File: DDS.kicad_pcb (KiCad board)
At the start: 4 copper layers, 70 x 100 mm, 175 parts, among them J1 Conn_01x05_Male, J2 USB_B_Mini, J3 Barrel_Jack_Switch, J4 Conn_Coaxial, J5 Conn_Coaxial, J6 Conn_Coaxial, U1 5M160ZT100, U2 LM317_SOT-223, U3 MCP2210x-SS, U4 ETXO-H33CL-100.000, U5 IS61LF12836, U6 DAC5687IPZP, Y1 12Meg

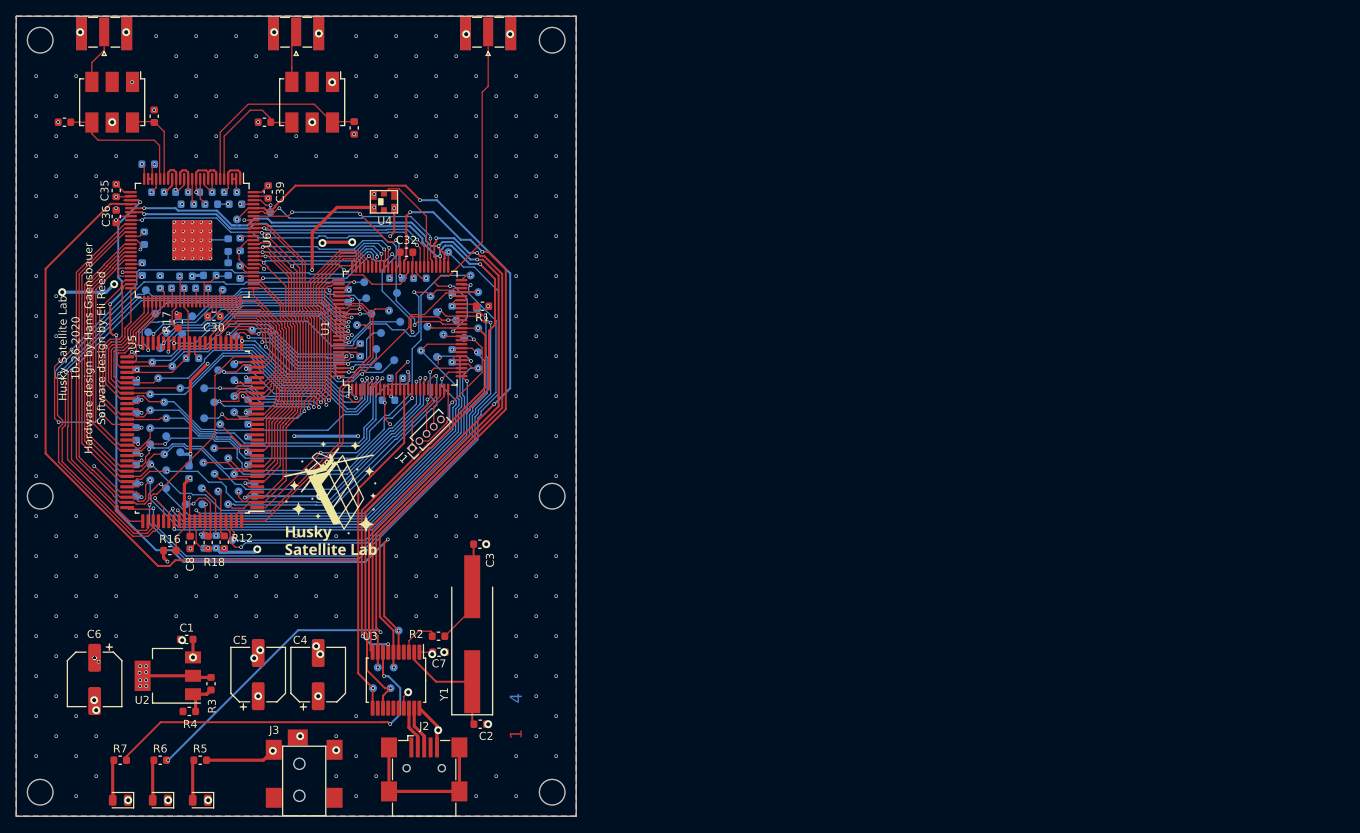
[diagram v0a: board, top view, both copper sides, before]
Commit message: new changes
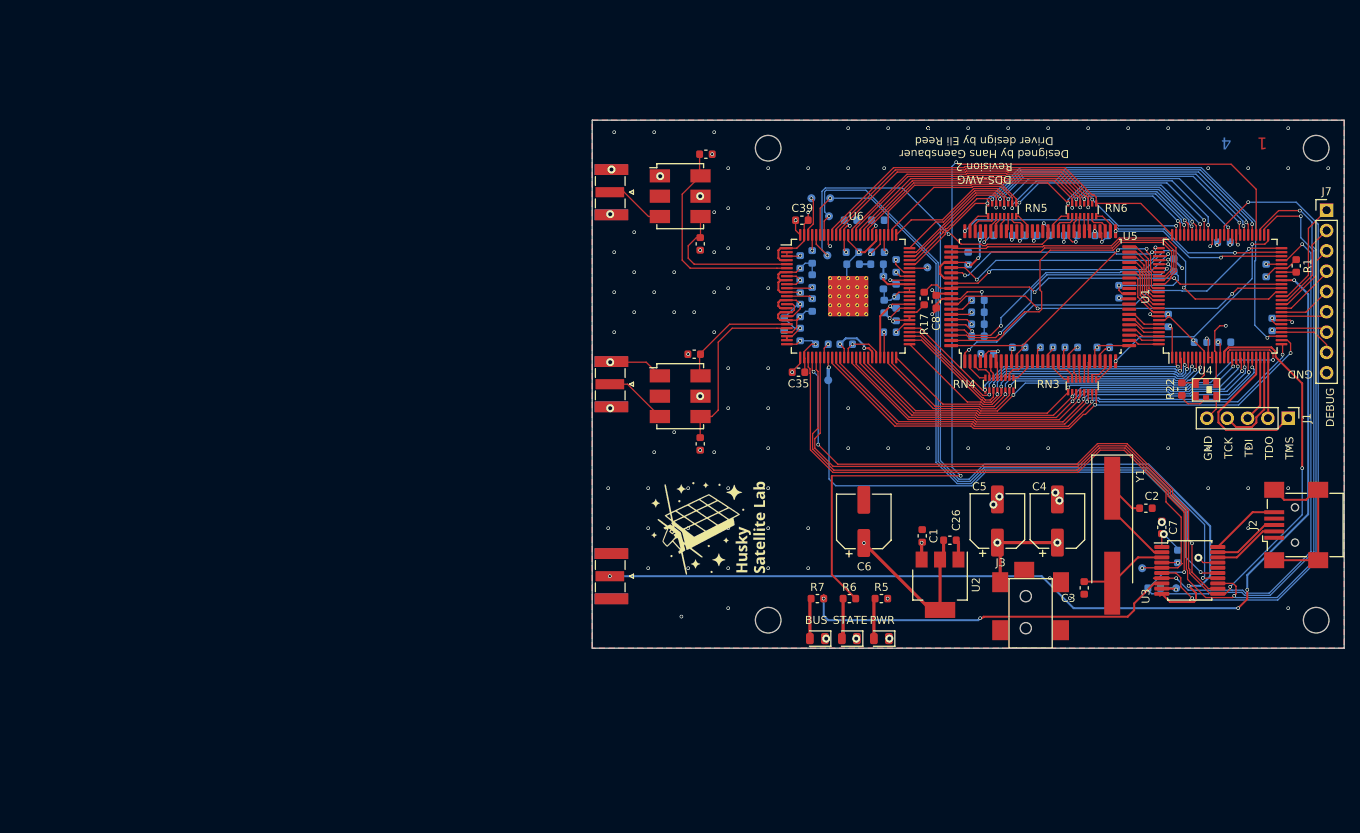
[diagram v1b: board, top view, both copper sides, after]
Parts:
- removed A0, A1, A10, A11, A12, A13, A14, A15, A16, A2, A3, A4, A5, A6, A7, A8, A9, CS_DAC, CS_MEM, D0, D10, D11, D12, D13, D14, D15, D16, D17, D18, D19, D20, D21, D22, D23, D24, D25, D26, D27, D28, D29, D30, D31, D4, D5, D6, D7, D8, D9, HSC, LSC, MISO, MOSI, SCK, TP26, TP27, TP28, TP29, TP30, TP31, TP32, TP34, TP37, TP39, TP40, TP41, TP42, TP43, TP46, TP47, TP48, TP49, TP7, ~CE: TestPoint, TestPoint:TestPoint_Pad_D1.0mm
- removed the D1 at (59.5, 103.8)
- removed the D2 at (57.8, 105.2)
- removed the D3 at (60.5, 106.5)
- removed the D3 at (53.0, 158.0)
- removed R14: 22, Resistor_SMD:R_0603_1608Metric
- removed R16: 1k, Resistor_SMD:R_0603_1608Metric
- removed R3: 510, Resistor_SMD:R_0603_1608Metric
- removed R4: 220, Resistor_SMD:R_0603_1608Metric
- removed REF** (x6): MountingHole_3.2mm_M3_DIN965, MountingHole:MountingHole_3.2mm_M3_DIN965
- added C26: 1u, Capacitor_SMD:C_0603_1608Metric, F.Cu at (156.7, 125.5)
- added D3: LED_Small, LED_SMD:LED_0805_2012Metric, F.Cu at (140.2, 137.8)
- added H1: MountingHole, MountingHole:MountingHole_3.2mm_M3, F.Cu at (134.0, 135.5)
- added H2: MountingHole, MountingHole:MountingHole_3.2mm_M3, F.Cu at (202.5, 135.5)
- added H3: MountingHole, MountingHole:MountingHole_3.2mm_M3, F.Cu at (134.0, 76.5)
- added H4: MountingHole, MountingHole:MountingHole_3.2mm_M3, F.Cu at (202.5, 76.5)
- added J7: Debug_Header, Connector_PinHeader_2.54mm:PinHeader_1x09_P2.54mm_Vertical, F.Cu at (203.8, 84.2)
- added R21: 1k, Resistor_SMD:R_0603_1608Metric, B.Cu at (185.2, 127.5)
- added R22: 1k, Resistor_SMD:R_0603_1608Metric, F.Cu at (185.7, 106.6)
- added RN3: R_Pack08, HS2_parts:CAY16-470J8LF, F.Cu at (173.2, 106.2)
- added RN4: R_Pack08, HS2_parts:CAY16-470J8LF, F.Cu at (162.9, 106.0)
- added RN5: R_Pack08, HS2_parts:CAY16-470J8LF, F.Cu at (163.2, 84.2)
- added RN6: R_Pack08, HS2_parts:CAY16-470J8LF, F.Cu at (173.2, 84.2)
- added TP1: TestPoint, TestPoint:TestPoint_Pad_D1.0mm, B.Cu at (185.0, 131.5)
- added TP5: TestPoint, TestPoint:TestPoint_Pad_D1.0mm, B.Cu at (180.8, 129.0)
- added TP9: TestPoint, TestPoint:TestPoint_Pad_D1.0mm, B.Cu at (141.8, 82.8)
- C30, C32, C36, R12, R18: moved to B.Cu
- J1: footprint Connector_PinHeader_1.27mm:PinHeader_1x05_P1.27mm_Vertical -> Connector_PinHeader_2.54mm:PinHeader_1x05_P2.54mm_Vertical
- R2: value 22 -> 100; moved to B.Cu
- U2: value LM317_SOT-223 -> AZ1117-1.8
- moved C15 121.9 mm to (175.6, 87.4), turned to 0 degrees
- moved C13 118.8 mm to (171.8, 87.4), turned to 180 degrees
- moved C17 116.1 mm to (177.8, 94.4), turned to 90 degrees
- moved C27 116.1 mm to (168.4, 87.4), turned to 0 degrees
- moved C43 115.6 mm to (197.0, 98.5), turned to 90 degrees
- moved C11 113.8 mm to (165.3, 87.4), turned to 0 degrees
- moved C44 113.7 mm to (196.2, 91.8)
- moved J2 113.0 mm to (199.8, 123.6), turned to 90 degrees
- moved C9 111.0 mm to (161.4, 87.4), turned to 180 degrees
- moved J1 109.6 mm to (199.0, 110.2), turned to 270 degrees
- moved U5 107.4 mm to (168.0, 95.0), turned to 90 degrees
- moved C19 106.9 mm to (175.9, 101.4), turned to 0 degrees
- moved U4 105.4 mm to (188.7, 106.7), turned to 180 degrees
- moved C31 104.8 mm to (191.0, 88.2), turned to 180 degrees
- moved C34 103.9 mm to (191.0, 100.8), turned to 180 degrees
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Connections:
- net Net-(J1-Pad1) renamed /TMS
- net Net-(J1-Pad2) renamed /TDO
- net Net-(J1-Pad3) renamed /TDI
- net Net-(J1-Pad4) renamed /TCK
- J2 pad 1: +5V -> (no net)
- J2 pad 4: Net-(J2-Pad4) -> (no net)
- R17 pad 2: /HS_CLK -> /SRAM_CLK
- R2 pad 2: Net-(C3-Pad1) -> /MOSI
- U1 pad 100: /A0 -> /A2
- U1 pad 29: /~ADSC -> Net-(J7-Pad8)
- U1 pad 30: /~OE -> Net-(J7-Pad7)
- U1 pad 33: /~BWE -> Net-(J7-Pad6)
- U1 pad 34: /~GW -> Net-(J7-Pad5)
- U1 pad 35: /~CE2 -> Net-(J7-Pad4)
- U1 pad 36: /LS_CLK -> Net-(J7-Pad3)
- U1 pad 37: /TRIG -> Net-(J7-Pad2)
- U1 pad 38: /IO2 -> Net-(J7-Pad1)
- U1 pad 39: /PHSTR -> /~GW
- U1 pad 40: /TXEN -> /~CE2
- U1 pad 41: /CE2 -> /SRAM_CLK
- U1 pad 42: /~CE -> /TRIG
- U1 pad 43: Net-(U1-Pad43) -> (no net)
- U1 pad 47: /MODE -> /IO2
- U1 pad 55: /DAC_RST -> /D17
- U1 pad 56: /HS_CLK_EN -> /D18
- U1 pad 57: /D17 -> /D19
- U1 pad 58: /D18 -> /D20
- U1 pad 61: /D19 -> /D21
- U1 pad 64: /ZZ -> (no net)
- U1 pad 66: /D20 -> /D22
- U1 pad 67: /D21 -> /D23
- U1 pad 68: /D22 -> /D24
- U1 pad 69: /D23 -> /D25
- U1 pad 70: /D24 -> /D26
- U1 pad 71: /D25 -> /D27
- U1 pad 72: /D26 -> /D28
- U1 pad 73: /D27 -> /D29
- U1 pad 74: /D28 -> /D30
- U1 pad 75: /D29 -> /D31
- U1 pad 76: /D30 -> /~ADSC
- U1 pad 77: /D31 -> /~OE
- U1 pad 78: /~ADV -> /CE2
- U1 pad 81: /~ADSP -> /~CE
- U1 pad 95: /A5 -> /A0
- U1 pad 96: /A4 -> /A1
- U1 pad 97: /A3 -> /A5
- U1 pad 98: /A2 -> /A4
- U1 pad 99: /A1 -> /A3
- U2 pad 1: Net-(R3-Pad1) -> AGND
- U3 pad 12: Net-(U3-Pad12) -> /DAC_RST
- U3 pad 14: Net-(U3-Pad14) -> /PHSTR
- U3 pad 15: Net-(U3-Pad15) -> /TXEN
- U3 pad 16: Net-(U3-Pad16) -> (no net)
- U3 pad 3: Net-(R2-Pad1) -> Net-(C3-Pad1)
- U3 pad 9: /MOSI -> Net-(R2-Pad1)
- U4 pad 1: Net-(U4-Pad1) -> (no net)
- U4 pad 2: /HS_CLK_EN -> Net-(R22-Pad1)
- U4 pad 5: Net-(U4-Pad5) -> (no net)
- U5 pad 12: /D22 -> Net-(RN4-Pad7)
- U5 pad 13: /D23 -> Net-(RN4-Pad8)
- U5 pad 14: Net-(U5-Pad14) -> (no net)
- U5 pad 16: Net-(U5-Pad16) -> (no net)
- U5 pad 18: /D24 -> Net-(RN3-Pad1)
- U5 pad 19: /D25 -> Net-(RN3-Pad2)
- U5 pad 2: /D16 -> Net-(RN4-Pad1)
- U5 pad 22: /D26 -> Net-(RN3-Pad3)
- U5 pad 23: /D27 -> Net-(RN3-Pad4)
- U5 pad 24: /D28 -> Net-(RN3-Pad5)
- U5 pad 25: /D29 -> Net-(RN3-Pad6)
- U5 pad 28: /D30 -> Net-(RN3-Pad7)
- U5 pad 29: /D31 -> Net-(RN3-Pad8)
- U5 pad 3: /D17 -> Net-(RN4-Pad2)
- U5 pad 31: /MODE -> AGND
- U5 pad 38: Net-(U5-Pad38) -> (no net)
- U5 pad 39: Net-(U5-Pad39) -> (no net)
- U5 pad 42: Net-(U5-Pad42) -> (no net)
- U5 pad 43: Net-(U5-Pad43) -> (no net)
- U5 pad 52: /D0 -> Net-(RN6-Pad1)
- U5 pad 53: /D1 -> Net-(RN6-Pad2)
- U5 pad 56: /D2 -> Net-(RN6-Pad3)
- U5 pad 57: /D3 -> Net-(RN6-Pad4)
- U5 pad 58: /D4 -> Net-(RN6-Pad5)
- U5 pad 59: /D5 -> Net-(RN6-Pad6)
- U5 pad 6: /D18 -> Net-(RN4-Pad3)
- U5 pad 62: /D6 -> Net-(RN6-Pad7)
- U5 pad 63: /D7 -> Net-(RN6-Pad8)
- U5 pad 64: /ZZ -> /SLEEP
- U5 pad 66: Net-(U5-Pad66) -> (no net)
- U5 pad 68: /D8 -> Net-(RN5-Pad1)
- U5 pad 69: /D9 -> Net-(RN5-Pad2)
- U5 pad 7: /D19 -> Net-(RN4-Pad4)
- U5 pad 72: /D10 -> Net-(RN5-Pad3)
- U5 pad 73: /D11 -> Net-(RN5-Pad4)
- U5 pad 74: /D12 -> Net-(RN5-Pad5)
- U5 pad 75: /D13 -> Net-(RN5-Pad6)
- U5 pad 78: /D14 -> Net-(RN5-Pad7)
- U5 pad 79: /D15 -> Net-(RN5-Pad8)
- U5 pad 8: /D20 -> Net-(RN4-Pad5)
- U5 pad 83: /~ADV -> +3V3
- U5 pad 84: /~ADSP -> +3V3
- U5 pad 87: /~BWE -> +3V3
- U5 pad 89: Net-(R14-Pad2) -> /SRAM_CLK
- U5 pad 9: /D21 -> Net-(RN4-Pad6)
- U6 pad 62: Net-(U6-Pad62) -> (no net)
- U6 pad 63: Net-(U6-Pad63) -> (no net)
- U6 pad 71: /D31 -> /D16
- U6 pad 72: /D30 -> /D17
- U6 pad 73: /D29 -> /D18
- U6 pad 74: /D28 -> /D19
- U6 pad 75: /D27 -> /D20
- U6 pad 76: /D26 -> /D21
- U6 pad 77: /D25 -> /D22
- U6 pad 78: /D24 -> /D23
- U6 pad 83: /D23 -> /D24
- U6 pad 84: /D22 -> /D25
- U6 pad 85: /D21 -> /D26
- U6 pad 86: /D20 -> /D27
- U6 pad 87: /D19 -> /D28
- U6 pad 90: /D18 -> /D29
- U6 pad 91: /D17 -> /D30
- U6 pad 92: /D16 -> /D31
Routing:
- net /TRIG: track 45.6 -> 127.1 mm, vias 2 -> 4
- net /DQPd: track 107.2 -> 28.6 mm
- net /HS_CLK: track 86.0 -> 8.29 mm, vias 6 -> 1
- net /~ADV: track 74.3 -> 0.00 mm, vias 2 -> 0
- net /~ADSP: track 71.0 -> 0.00 mm, vias 2 -> 0
- net /ZZ: track 69.1 -> 0.00 mm, vias 4 -> 0
- net /DAC_RST: track 28.1 -> 93.9 mm
- net /PHSTR: track 37.9 -> 95.4 mm, vias 4 -> 2
- net /~BWE: track 56.2 -> 0.00 mm, vias 2 -> 0
- net /LS_CLK: track 51.1 -> 0.00 mm, vias 2 -> 0
- net /SRAM_CLK: track 0.00 -> 46.6 mm, vias 0 -> 2
- net +1V8: track 236.4 -> 194.2 mm, vias 24 -> 13
- net /MOSI: track 109.6 -> 149.3 mm, vias 4 -> 2
- net /MODE: track 39.5 -> 0.00 mm, vias 3 -> 0
- net AGND: track 106.4 -> 145.7 mm, vias 251 -> 136
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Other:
- board size 70 x 100 mm -> 94 x 66 mm
- board text added: "BUS"
- board text added: "CS_DAC"
- board text added: "DDS-AWG Revision 2 Designed by Hans Gaensbauer Driver design by Eli Reed"
- board text added: "DEBUG"
- board text added: "GND"
- board text added: "PHSTR"
- board text added: "PLLLOCK"
- board text added: "PWR"
- board text added: "QFLG"
- board text added: "RST"
- board text added: "SDIO_MCP"
- board text added: "SLEEP"
- board text added: "STATE"
- board text added: "TCK"
- board text added: "TDI"
- board text added: "TDO"
- board text added: "TMS"
- board text added: "TRIG"
- board text added: "TXEN"
- board text removed: "Husky Satellite Lab 10-26-2020 Hardware design by Hans Gaensbauer Software design by Eli Reed"
